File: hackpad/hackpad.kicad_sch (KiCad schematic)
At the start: 10 parts, among them SW1 SW_Push, SW10 SW_Push, SW2 SW_Push, SW3 SW_Push, SW4 SW_Push, SW5 SW_Push, SW6 SW_Push, SW7 SW_Push, SW9 SW_Push, U1 MOUDLE-SEEEDUINO-XIAO

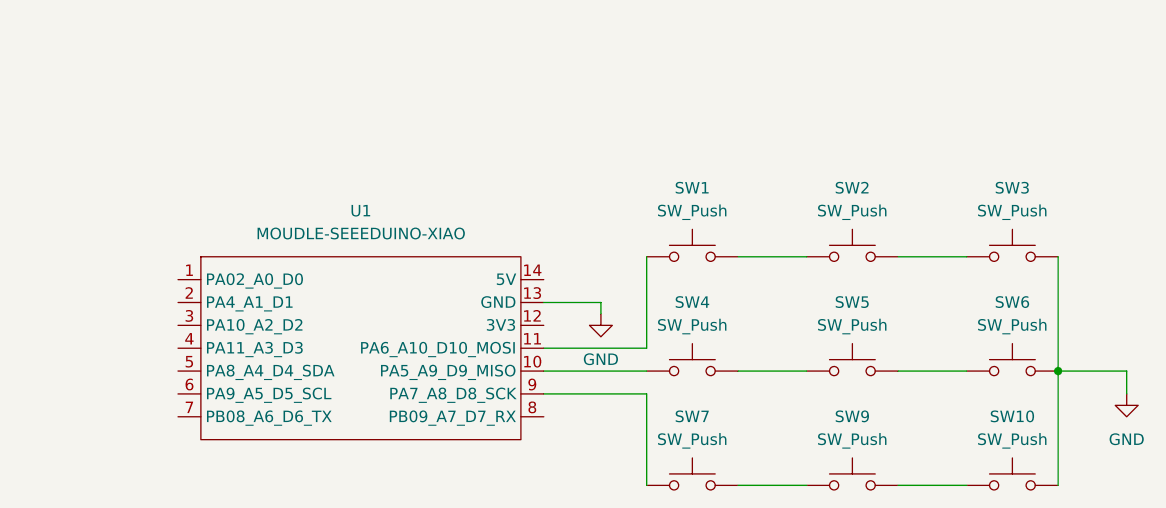
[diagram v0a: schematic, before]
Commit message: Update
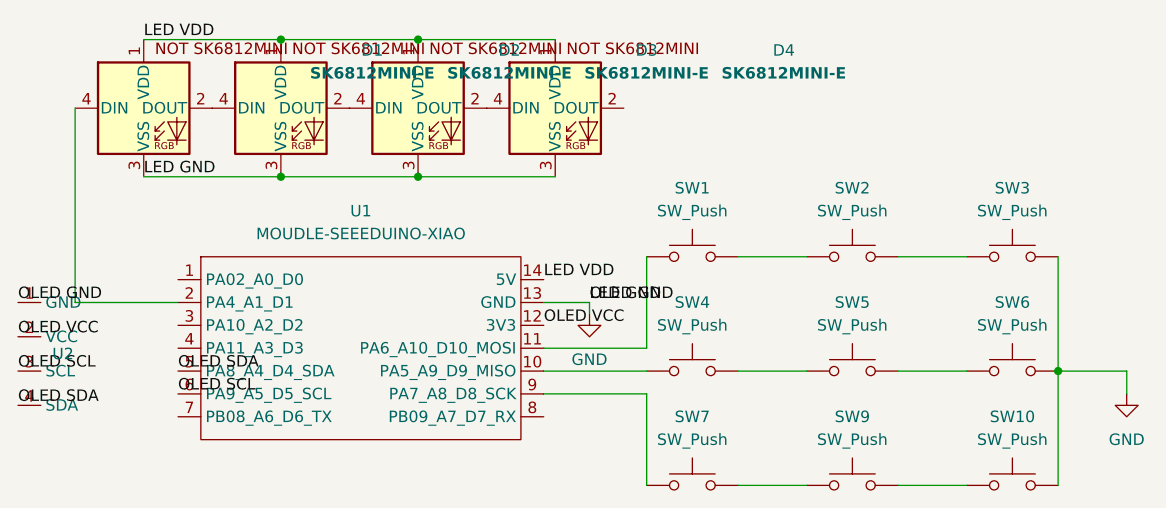
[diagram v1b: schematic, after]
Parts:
- added D1, D2, D3, D4: SK6812MINI-E, footprints:SK6812MINI-E_fixed, symbol SK6812MINI-E:SK6812MINI-E
- added U2: (no value), OLED:SSD1306-0.91-OLED-4pin-128x32, symbol XIAO_RP2040:OLED_0.91_I2C_
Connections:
- net GND: now also D1.3 (VSS), D2.3 (VSS), D3.3 (VSS), D4.3 (VSS), U2.1 (GND)
- net OLED VCC: now reaches U1.12 (3V3)
- net OLED VCC: now also U2.2 (VCC)
- net LED VDD: now reaches U1.14 (5V)
- net LED VDD: now also D1.1 (VDD), D2.1 (VDD), D3.1 (VDD), D4.1 (VDD)
- net at U1.2 (PA4_A1_D1): now also D1.4 (DIN)
- net at U1.5 (PA8_A4_D4_SDA): no longer names the net of U1.5 (PA8_A4_D4_SDA)
- net at U1.5 (PA8_A4_D4_SDA): now also U2.4 (SDA)
- net OLED SCL: now reaches U1.6 (PA9_A5_D5_SCL)
- net OLED SCL: now also U2.3 (SCL)
- new net: D3.2 (DOUT), D4.4 (DIN)
- new net: D1.2 (DOUT), D2.4 (DIN)
- new net: D2.2 (DOUT), D3.4 (DIN)
